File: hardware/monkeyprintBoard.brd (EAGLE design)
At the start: 65 x 55.9 mm, 46 parts, among them Q1 BSS123

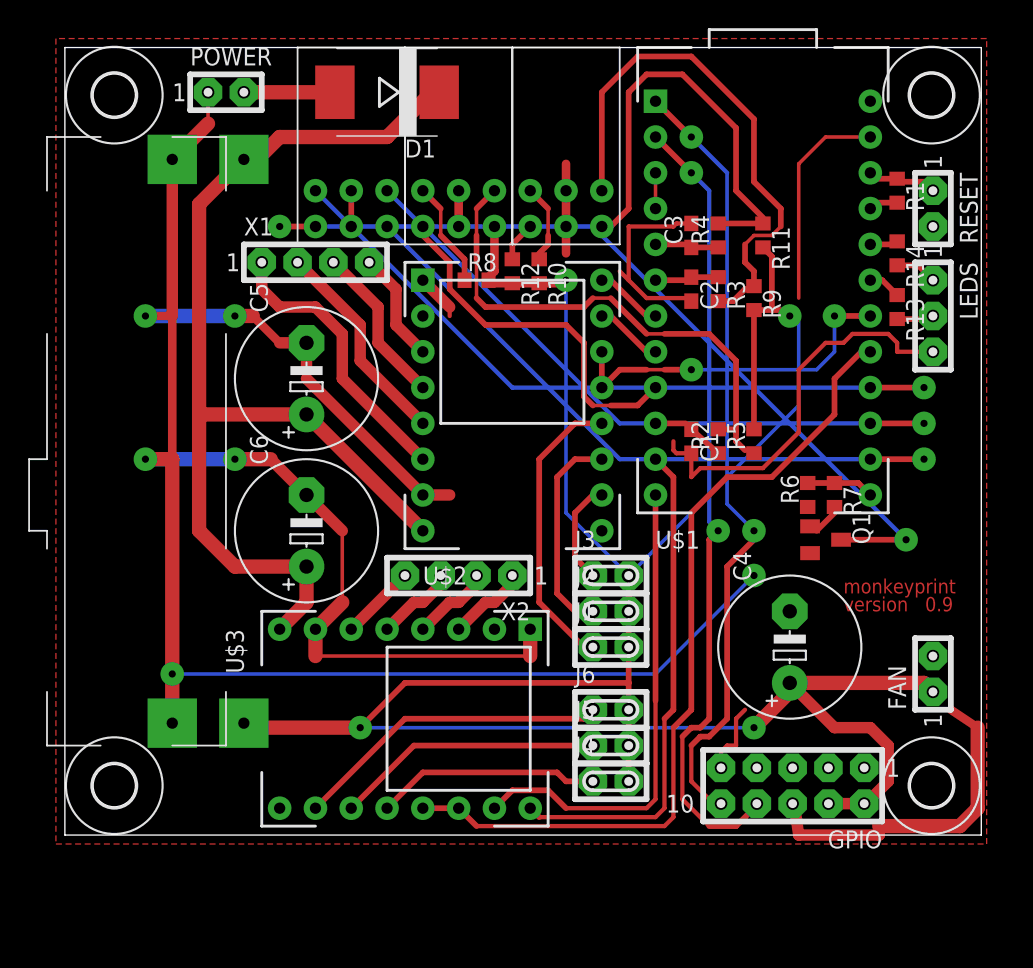
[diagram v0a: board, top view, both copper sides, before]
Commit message: Updated eagle files.
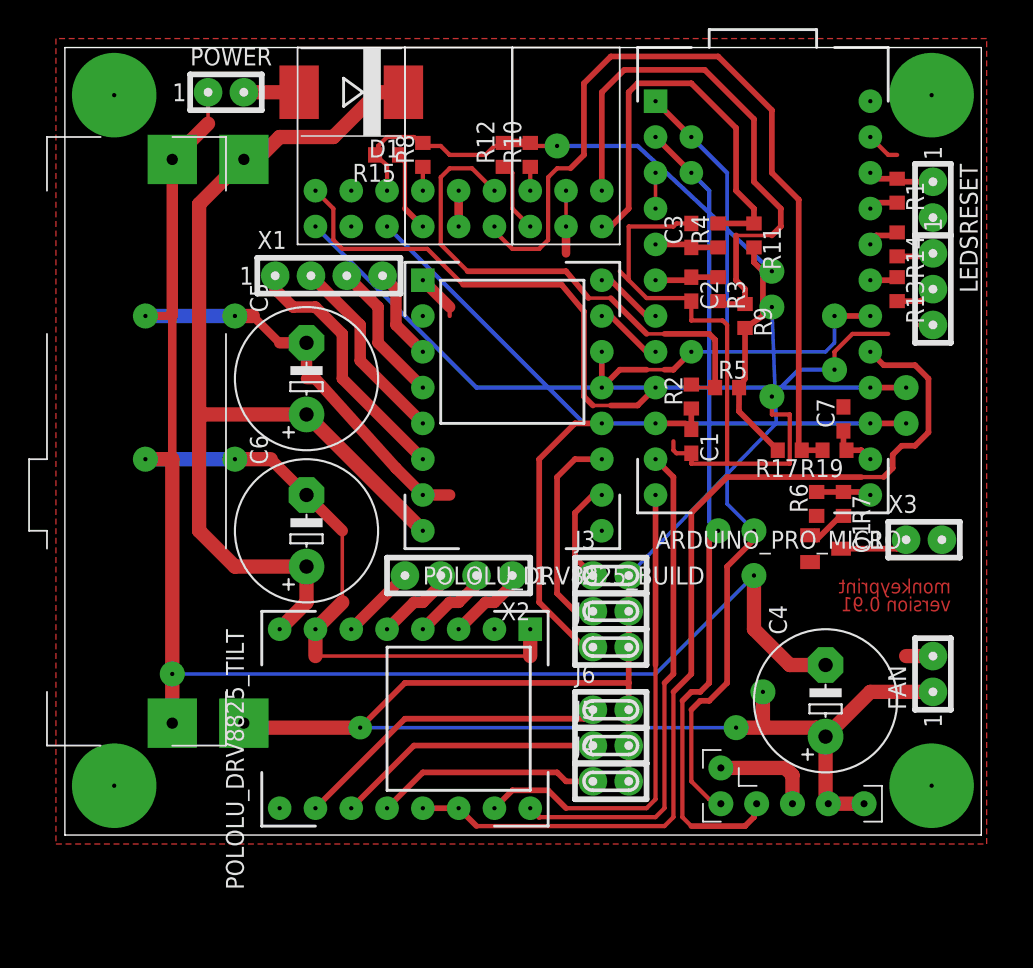
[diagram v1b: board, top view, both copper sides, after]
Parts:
- removed GPIO: (no value), connectors:X10N-DIL
- removed H1, H2, H3, H4: MOUNT-HOLE3.0, holes:3,0
- added ARDUINO_PRO_MICRO: ARDUINOPROMICRO, arduinoProMicro:ARDUINOPROMICRO
- added C7: 100n, rcl:C0603
- added R15: 220R, rcl:R0603
- added R17: 10k, rcl:R0603
- added R19: 0R, rcl:R0603
- added X3: (no value), connectors:X02N-SIL
- U$1: value ARDUINOPROMICRO -> MONKEYPRINTPICONNECTOR; device arduinoProMicro:ARDUINOPROMICRO -> monkeyprintPiConnector:MONKEYPRINTPICONNECTOR
- moved U$1 35.9 mm to (51.6, 3.49)
- moved R8 9.67 mm to (25.4, 48.3), turned to 90 degrees
- moved R10 8.28 mm to (33.0, 48.3), turned to 90 degrees
- moved R12 8.28 mm to (31.1, 48.3), turned to 90 degrees
- moved C4 4.58 mm to (54.0, 9.53)
- moved R5 4.26 mm to (47.0, 31.8), turned to 0 degrees
- moved R2 3.70 mm to (44.5, 31.1)
- moved D1 2.54 mm to (20.3, 52.7)
- moved LEDS 1.91 mm to (61.6, 38.7)
- moved R9 1.42 mm to (48.3, 36.8)
- moved X1 1.35 mm to (18.7, 39.7)
- moved R13 1.27 mm to (59.1, 38.7)
- moved R6 0.90 mm to (53.3, 23.5)
- moved R7 0.90 mm to (55.2, 23.5)
- moved Q1 0.63 mm to (54.0, 20.3)
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- renumbered U$2 to POLOLU_DRV8825_BUILD, U$3 to POLOLU_DRV8825_TILT
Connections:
- new net N$49: R17.1, R19.2, U$6.6
- new net N$50: ARDUINO_PRO_MICRO.14, C7.1, R19.1
- net GND: now also ARDUINO_PRO_MICRO.23, ARDUINO_PRO_MICRO.3, ARDUINO_PRO_MICRO.4, C7.2, U$1.GND1, U$1.GND2, X3.2; no longer GPIO.6, GPIO.9, U$1.23, U$1.3, U$1.4
- net N$1: now also ARDUINO_PRO_MICRO.7; no longer U$1.7
- net N$12: now also ARDUINO_PRO_MICRO.5; no longer U$1.5
- net N$13: now also ARDUINO_PRO_MICRO.6; no longer U$1.6
- net N$2: now also ARDUINO_PRO_MICRO.8; no longer U$1.8
- net N$25: now also ARDUINO_PRO_MICRO.10; no longer U$1.10
- net N$26: now also ARDUINO_PRO_MICRO.1, U$1.RXD; no longer GPIO.10, U$1.1
- net N$27: now also ARDUINO_PRO_MICRO.13; no longer U$1.13
- net N$28: now also ARDUINO_PRO_MICRO.22; no longer U$1.22
- net N$29: now also ARDUINO_PRO_MICRO.16, U$7.4; no longer U$1.16, U$7.1
- net N$31: now also X3.1; no longer U$7.4
- net N$32: now also ARDUINO_PRO_MICRO.19; no longer U$1.19
- net N$33: now also ARDUINO_PRO_MICRO.21; no longer U$1.21
- net N$34: now also ARDUINO_PRO_MICRO.20; no longer U$1.20
- net N$37: now also ARDUINO_PRO_MICRO.2, U$1.TXD; no longer GPIO.8, U$1.2
- net N$38: now also ARDUINO_PRO_MICRO.15, U$7.6; no longer U$1.15, U$7.3
- net N$39: now also ARDUINO_PRO_MICRO.9, U$7.1; no longer U$1.9, U$6.4
- net N$4: now also ARDUINO_PRO_MICRO.12; no longer U$1.12
- net N$41: now also R15.1, U$6.4; no longer U$1.14, U$7.6
- net N$5: now also ARDUINO_PRO_MICRO.18; no longer U$1.18
- net N$6: now also ARDUINO_PRO_MICRO.11; no longer U$1.11
- net N$8: now also ARDUINO_PRO_MICRO.17; no longer U$1.17
- net VCC: now also R15.2, R17.2, U$1.VCC1, U$1.VCC2, U$7.3; no longer GPIO.2, GPIO.4, U$6.6
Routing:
- net N$49: track 0.00 -> 59.8 mm
- net N$31: track 60.8 -> 4.88 mm, vias 2 -> 0
- net N$41: track 49.4 -> 5.75 mm, vias 1 -> 0
- net GND: track 273.5 -> 256.0 mm, vias 6 -> 8
- net N$39: track 26.0 -> 35.9 mm
- net N$8: track 59.6 -> 69.2 mm
- net N$10: track 7.58 -> 1.69 mm
- net N$11: track 5.65 -> 1.69 mm
- net N$38: track 48.7 -> 45.2 mm
- net N$29: track 52.8 -> 49.2 mm
- net N$50: track 0.00 -> 3.54 mm
- net N$14: track 2.85 -> 5.94 mm
- net N$40: track 6.46 -> 3.92 mm
- net V+: track 57.4 -> 54.9 mm
- net VCC: track 175.7 -> 173.8 mm, vias 4 -> 5
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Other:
- board text added: "version 0.91"
